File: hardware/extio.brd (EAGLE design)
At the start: 100 x 80 mm, 45 parts, among them IC1 PCF8574P, Q1 IRLZ44N, Q2 IRLZ44N, Q3 IRLZ44N, Q4 IRLZ44N, Q5 IRLZ44N, Q6 IRLZ44N, Q7 IRLZ44N, Q8 IRLZ44N

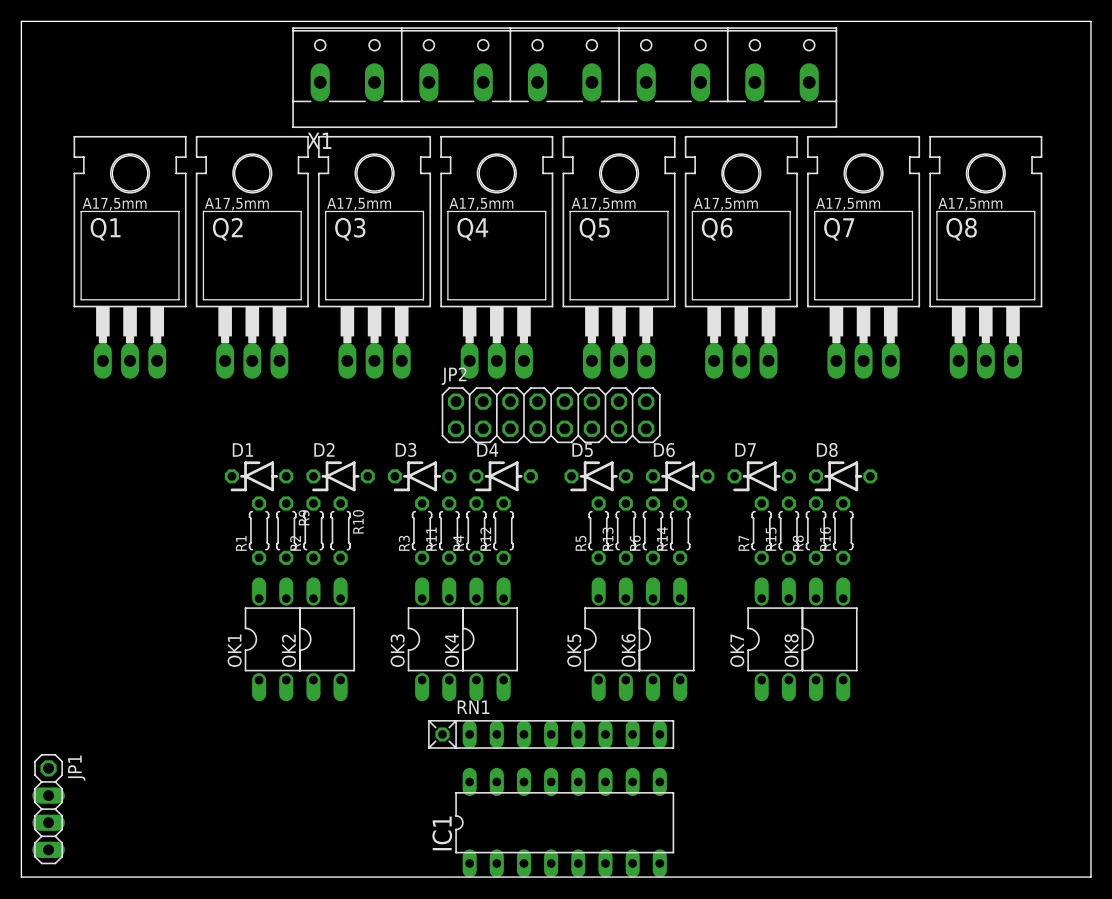
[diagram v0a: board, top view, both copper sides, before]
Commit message: extio board
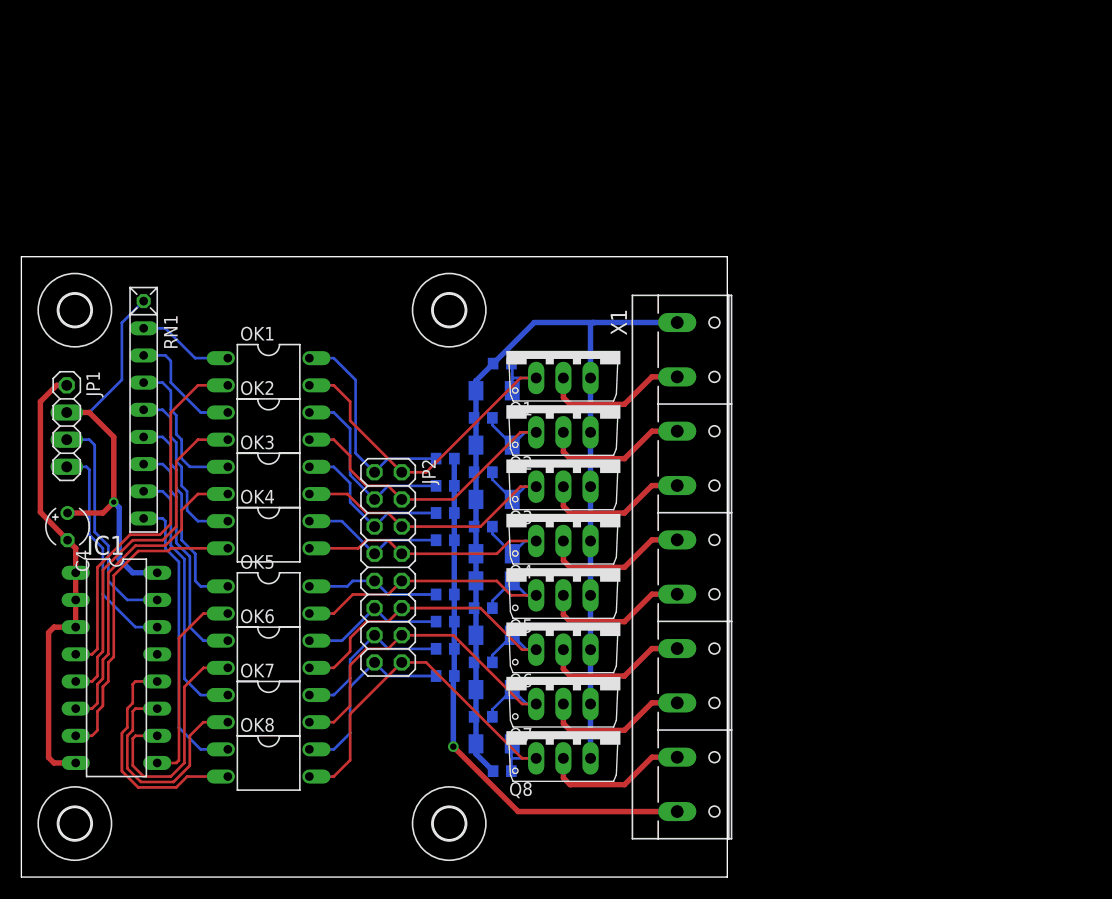
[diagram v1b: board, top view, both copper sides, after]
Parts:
- added C4: 1uF, resistor:TT2D4
- added U$1, U$2, U$3, U$4: (no value), gate433:3,0
- D1, D2, D3, D4, D5, D6, D7, D8: device gate433:ZDIO-5 -> gate433:SOD80C
- Q1, Q2, Q3, Q4, Q5, Q6, Q7, Q8: device gate433:TO220BH -> gate433:TO220V
- R1, R10, R11, R12, R13, R14, R15, R16, R2, R3, R4, R5, R6, R7, R8, R9: device resistor:0204/5 -> resistor:R0603
- moved Q8 56.9 mm to (50.7, 13.6)
- moved OK8 53.7 mm to (23.1, 10.7), turned to 270 degrees
- moved RN1 48.7 mm to (11.4, 43.7), turned to 270 degrees
- moved OK7 47.8 mm to (23.1, 15.7), turned to 270 degrees
- moved X1 47.3 mm to (62.0, 29.0), turned to 270 degrees
- moved Q7 45.6 mm to (50.7, 18.7)
- moved IC1 44.3 mm to (8.89, 19.6), turned to 270 degrees
- moved D8 41.1 mm to (44.2, 12.4), flipped to the bottom
- moved Q1 40.9 mm to (50.7, 49.2)
- moved R16 39.0 mm to (45.0, 9.91), flipped to the bottom, turned to 180 degrees
- moved R8 37.2 mm to (39.6, 18.8), flipped to the bottom, turned to 180 degrees
- moved OK6 37.2 mm to (23.1, 20.8), turned to 270 degrees
- moved JP1 35.9 mm to (4.24, 42.2)
- moved Q6 35.0 mm to (50.7, 23.8)
- moved R15 33.5 mm to (43.2, 15.0), flipped to the bottom, turned to 180 degrees
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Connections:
- removed net N$58: X1.10
- net +12V: now also X1.10
- net N$20: now also Q1.2; no longer Q1.D
- net N$54: now also Q1.1; no longer Q1.G
- net N$57: now also Q2.1; no longer Q2.G
- net N$60: now also Q3.1; no longer Q3.G
- net N$61: now also Q4.1; no longer Q4.G
- net N$62: now also Q5.1; no longer Q5.G
- net N$63: now also Q6.1; no longer Q6.G
- net N$65: now also Q7.1; no longer Q7.G
- net N$66: now also Q8.1; no longer Q8.G
- net N$67: now also Q2.2; no longer Q2.D
- net N$69: now also C4.+
- net N$71: now also C4.-
- net N$72: now also Q3.2; no longer Q3.D
- net N$77: now also Q4.2; no longer Q4.D
- net N$81: now also Q5.2; no longer Q5.D
- net N$85: now also Q6.2; no longer Q6.D
- net N$89: now also Q7.2; no longer Q7.D
- net N$93: now also Q8.2; no longer Q8.D
- net PE: now also Q1.3, Q2.3, Q3.3, Q4.3, Q5.3, Q6.3, Q7.3, Q8.3; no longer Q1.S, Q2.S, Q3.S, Q4.S, Q5.S, Q6.S, Q7.S, Q8.S
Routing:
- net PE: track 0.00 -> 100.1 mm
- net +12V: track 0.00 -> 50.4 mm, vias 0 -> 1
- net N$71: track 0.00 -> 42.7 mm
- net N$69: track 0.00 -> 40.4 mm, vias 0 -> 1
- net N$66: track 0.00 -> 36.8 mm
- net N$65: track 0.00 -> 35.6 mm
- net N$46: track 0.00 -> 35.2 mm
- net N$54: track 0.00 -> 34.1 mm
- net N$57: track 0.00 -> 32.9 mm
- net N$45: track 0.00 -> 32.7 mm
- net N$63: track 0.00 -> 32.0 mm
- net N$44: track 0.00 -> 30.1 mm
- net N$60: track 0.00 -> 30.1 mm
- net N$62: track 0.00 -> 29.1 mm
- net N$43: track 0.00 -> 29.1 mm
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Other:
- board size 100 x 80 mm -> 66 x 58 mm

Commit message: extio.brd, mainboard.brd, gate433.lib
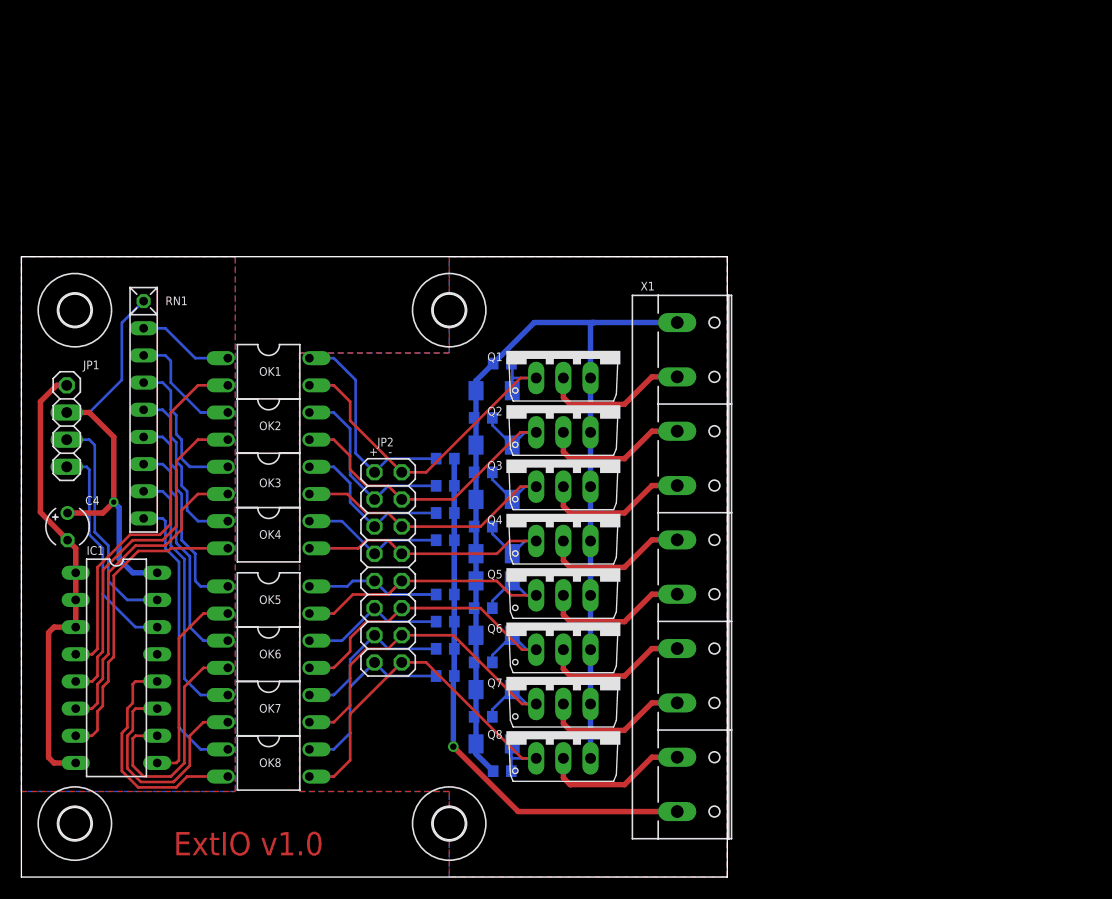
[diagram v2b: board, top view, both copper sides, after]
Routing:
- added copper zone on layer 1, net N$71
- added copper zone on layer 16, net N$71
- added copper zone on layer 1, net PE
- added copper zone on layer 16, net PE
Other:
- board text added: "+ -"
- board text added: "ExtIO v1.0"
